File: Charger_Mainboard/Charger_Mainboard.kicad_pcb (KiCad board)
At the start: 2 copper layers, 100 x 100 mm, 57 parts, among them J1 Conn_01x02, J10 Conn_02x10_Odd_Even, J11 Conn_01x02_Pin, J12 Conn_01x02_Pin, J13 Conn_01x02_Pin, J14 Conn_01x02_Pin, J15 Conn_01x02_Pin, J16 Conn_01x02_Pin, J17 Conn_01x02_Pin, J18 Conn_01x04, J19 Conn_01x02_Pin, J2 Conn_01x02, J20 Conn_01x02_Pin, J21 Conn_01x04, J22 Conn_01x04, J23 Conn_01x02_Pin, J24 Conn_01x02_Pin, J3 Conn_01x02, J4 Conn_01x02, J5 Conn_01x02, J6 Conn_01x02, J7 Conn_01x02, J8 Conn_01x04, J9 Conn_01x02_Pin, U1 AP2204K-ADJ, U2 TLV2371DBV, U3 AP2204K-ADJ

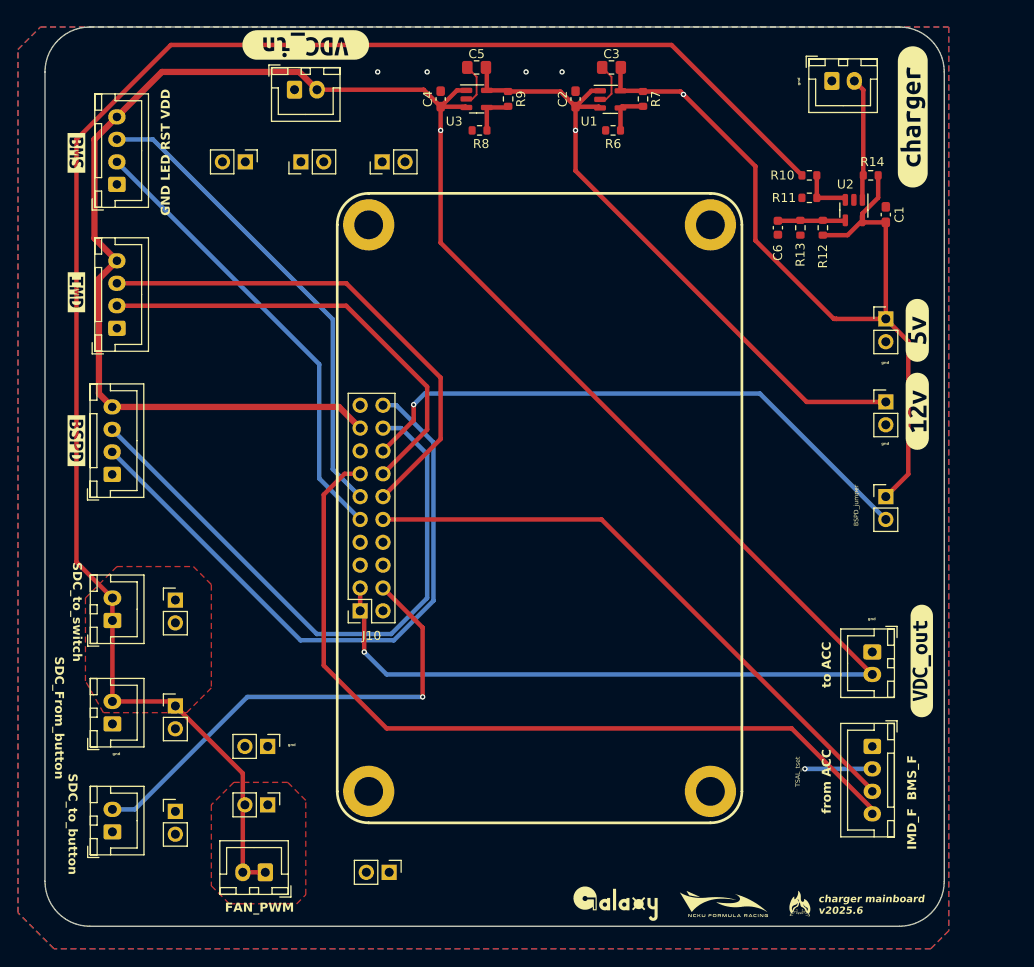
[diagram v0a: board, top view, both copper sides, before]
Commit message: Charger v2026.1
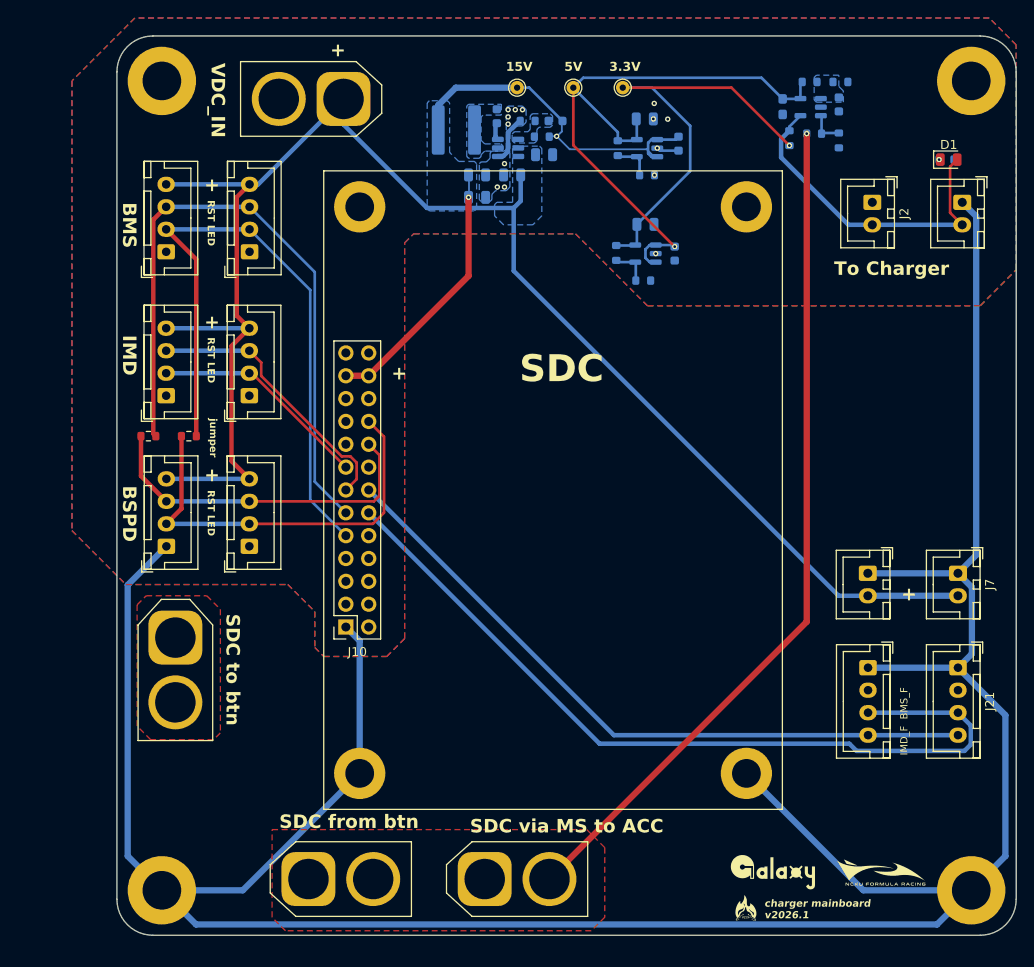
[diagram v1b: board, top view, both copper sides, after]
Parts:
- removed the H1 at (156.0, 65.0)
- removed the H2 at (118.0, 128.0)
- removed the H3 at (156.0, 128.0)
- removed the H4 at (118.0, 65.0)
- removed J11, J12, J13, J14, J15, J16, J17, J19, J20, J23, J24, J9: Conn_01x02_Pin, Connector_PinHeader_2.54mm:PinHeader_1x02_P2.54mm_Vertical
- removed the J18 at (90.0, 76.5)
- removed the J2 at (169.5, 49.0)
- removed the J21 at (174.0, 123.0)
- removed the J22 at (90.0, 60.5)
- removed J6: Conn_01x02, Connector_JST:JST_XH_B2B-XH-A_1x02_P2.50mm_Vertical
- removed the J7 at (174.0, 112.5)
- removed the J8 at (89.5, 92.8)
- removed kibuzzard-682D8AF9: G***, kibuzzard-682D8AF9
- removed kibuzzard-682D8B7A: G***, kibuzzard-682D8B7A
- removed kibuzzard-68452BF1: G***, kibuzzard-68452BF1
- removed kibuzzard-68452CD9: G***, kibuzzard-68452CD9
- removed kibuzzard-68452D38: G***, kibuzzard-68452D38
- removed kibuzzard-68452D90: G***, kibuzzard-68452D90
- removed kibuzzard-684531AC: G***, kibuzzard-684531AC
- removed kibuzzard-68453814: G***, kibuzzard-68453814
- added C10: 22u, Capacitor_SMD:C_0805_2012Metric, B.Cu at (130.1, 62.0)
- added C11: 1u, Capacitor_SMD:C_0603_1608Metric, B.Cu at (152.0, 68.2)
- added C12: 10u, Capacitor_SMD:C_0805_2012Metric, B.Cu at (148.8, 65.0)
- added C7: 100n, Capacitor_SMD:C_0603_1608Metric, B.Cu at (132.2, 52.9)
- added C8: 12p, Capacitor_SMD:C_0603_1608Metric, B.Cu at (138.8, 53.5)
- added C9: 22u, Capacitor_SMD:C_0805_2012Metric, B.Cu at (130.1, 59.5)
- added D1: LED_Small, LED_SMD:LED_0805_2012Metric, F.Cu at (182.5, 57.8)
- added H1: MountingHole_Pad, MountingHole:MountingHole_4.3mm_M4_ISO7380_Pad, F.Cu at (185.0, 49.0)
- added H1: MountingHole_Pad, MountingHole:MountingHole_3.2mm_M3_ISO7380_Pad, F.Cu at (160.0, 63.0)
- added H2: MountingHole_Pad, MountingHole:MountingHole_3.2mm_M3_ISO7380_Pad, F.Cu at (117.0, 126.0)
- added H2: MountingHole_Pad, MountingHole:MountingHole_4.3mm_M4_ISO7380_Pad, F.Cu at (185.0, 139.0)
- added H3: MountingHole_Pad, MountingHole:MountingHole_4.3mm_M4_ISO7380_Pad, F.Cu at (95.0, 49.0)
- added H3: MountingHole_Pad, MountingHole:MountingHole_3.2mm_M3_ISO7380_Pad, F.Cu at (160.0, 126.0)
- added H4: MountingHole_Pad, MountingHole:MountingHole_3.2mm_M3_ISO7380_Pad, F.Cu at (117.0, 63.0)
- added H4: MountingHole_Pad, MountingHole:MountingHole_4.3mm_M4_ISO7380_Pad, F.Cu at (95.0, 139.0)
- added J18: Conn_01x04, Connector_JST:JST_XH_B4B-XH-A_1x04_P2.50mm_Vertical, F.Cu at (104.7, 84.0)
- added J18: Conn_01x04, Connector_JST:JST_XH_B4B-XH-A_1x04_P2.50mm_Vertical, F.Cu at (95.5, 84.0)
- added J2: Conn_01x02, Connector_JST:JST_XH_B2B-XH-A_1x02_P2.50mm_Vertical, F.Cu at (174.0, 62.5)
- added J2: Conn_01x02, Connector_JST:JST_XH_B2B-XH-A_1x02_P2.50mm_Vertical, F.Cu at (184.0, 62.5)
- added J21: Conn_01x04, Connector_JST:JST_XH_B4B-XH-A_1x04_P2.50mm_Vertical, F.Cu at (183.5, 114.2)
- added J21: Conn_01x04, Connector_JST:JST_XH_B4B-XH-A_1x04_P2.50mm_Vertical, F.Cu at (173.5, 114.2)
- added J22: Conn_01x04, Connector_JST:JST_XH_B4B-XH-A_1x04_P2.50mm_Vertical, F.Cu at (104.8, 68.0)
- added J22: Conn_01x04, Connector_JST:JST_XH_B4B-XH-A_1x04_P2.50mm_Vertical, F.Cu at (95.5, 68.0)
- added J7: Conn_01x02, Connector_JST:JST_XH_B2B-XH-A_1x02_P2.50mm_Vertical, F.Cu at (183.5, 103.8)
- added J7: Conn_01x02, Connector_JST:JST_XH_B2B-XH-A_1x02_P2.50mm_Vertical, F.Cu at (173.5, 103.8)
- added J8: Conn_01x04, Connector_JST:JST_XH_B4B-XH-A_1x04_P2.50mm_Vertical, F.Cu at (95.5, 100.8)
- added J8: Conn_01x04, Connector_JST:JST_XH_B4B-XH-A_1x04_P2.50mm_Vertical, F.Cu at (104.7, 100.8)
- added L1: 15uH, Inductor_SMD:L_Coilcraft_XAL6060-XXX, B.Cu at (127.8, 54.5)
- added R1: 0, Resistor_SMD:R_0603_1608Metric, F.Cu at (93.5, 88.5)
- added R2: 0, Resistor_SMD:R_0603_1608Metric, F.Cu at (98.0, 88.5)
- added R3: 301k, Resistor_SMD:R_0603_1608Metric, B.Cu at (167.5, 54.9)
- added R4: 100k, Resistor_SMD:R_0603_1608Metric, B.Cu at (170.3, 55.6)
- added R5: 10k, Resistor_SMD:R_0603_1608Metric, B.Cu at (182.2, 57.8)
- added TP1: TestPoint, TestPoint:TestPoint_THTPad_D1.5mm_Drill0.7mm, F.Cu at (134.5, 49.8)
- added TP2: TestPoint, TestPoint:TestPoint_THTPad_D1.5mm_Drill0.7mm, F.Cu at (140.8, 49.8)
- added TP3: TestPoint, TestPoint:TestPoint_THTPad_D1.5mm_Drill0.7mm, F.Cu at (146.2, 49.8)
- added U4: AP2204K-ADJ, Package_TO_SOT_SMD:SOT-23-5, B.Cu at (148.8, 68.2)
- C1, C6, R12, R13, R14, R6, R7, U1: moved to B.Cu
- C2: footprint Capacitor_SMD:C_0603_1608Metric_Pad1.08x0.95mm_HandSolder -> Capacitor_SMD:C_0603_1608Metric; moved to B.Cu
- C3, C5: footprint Capacitor_SMD:C_0805_2012Metric_Pad1.18x1.45mm_HandSolder -> Capacitor_SMD:C_0805_2012Metric; moved to B.Cu
- C4: value 1u -> 10u; footprint Capacitor_SMD:C_0603_1608Metric_Pad1.08x0.95mm_HandSolder -> Capacitor_SMD:C_0805_2012Metric; moved to B.Cu
- J1, J3, J4, J5: footprint Connector_JST:JST_XH_B2B-XH-A_1x02_P2.50mm_Vertical -> Connector_AMASS:AMASS_XT60-M_1x02_P7.20mm_Vertical
- J10: value Conn_02x10_Odd_Even -> Conn_02x13_Odd_Even; footprint Connector_PinSocket_2.54mm:PinSocket_2x10_P2.54mm_Vertical -> Connector_PinSocket_2.54mm:PinSocket_2x13_P2.54mm_Vertical
- R10: value 100R -> 100k; moved to B.Cu
- R11: value 100k -> 165k; moved to B.Cu
- R8: value 100k -> 534k; moved to B.Cu
- R9: value 301k -> 30k1; moved to B.Cu
- U2: value TLV2371DBV -> AS331KTR-G1; moved to B.Cu
- U3: value AP2204K-ADJ -> AP63200WU; footprint Package_TO_SOT_SMD:SOT-23-5 -> Package_TO_SOT_SMD:TSOT-23-6; moved to B.Cu
- moved J5 50.4 mm to (130.9, 137.8), turned to 0 degrees
- moved J4 27.8 mm to (111.3, 137.8), turned to 0 degrees
- moved J3 22.7 mm to (96.5, 110.9), turned to -90 degrees
- moved R11 22.3 mm to (145.5, 68.1), turned to -90 degrees
- moved R10 21.9 mm to (148.5, 71.2), turned to 180 degrees
- moved G*** 17.8 mm to (175.0, 137.0)
- moved G*** 17.8 mm to (163.0, 137.0)
- moved R13 16.8 mm to (170.5, 49.1), turned to 0 degrees
- moved C1 16.6 mm to (164.0, 51.9), turned to -90 degrees
- moved R12 16.3 mm to (167.0, 49.1), turned to 0 degrees
- moved C6 15.3 mm to (170.3, 51.6)
- moved C4 13.1 mm to (137.5, 57.2), turned to 0 degrees
- moved C5 12.6 mm to (133.9, 59.5)
- moved C2 12.5 mm to (152.4, 56.0), turned to -90 degrees
- moved U2 12.4 mm to (167.1, 51.9), turned to 180 degrees
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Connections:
- C2 pad 1: +12V -> SDC_IN
- C4 pad 1: BSPD_IN -> VDC
- C5 pad 1: +12V -> VDC
- J1 pad 1: GND -> VDC
- J1 pad 2: BSPD_IN -> GND
- J10 pad 1: BSPD_IN -> GND
- J10 pad 10: BMS_FAULT -> SDC_OUT
- J10 pad 12: IMD_RST -> BMS_FAULT
- J10 pad 13: IMD_FAULT -> IMD_RST
- J10 pad 14: IMD_LED -> IMD_FAULT
- J10 pad 15: GND -> IMD_LED
- J10 pad 16: BSPD_FAULT -> unconnected-(J10-Pin_16-Pad16)
- J10 pad 17: BSPD_IN -> BSPD_FAULT
- J10 pad 2: GND -> unconnected-(J10-Pin_2-Pad2)
- J10 pad 3: BSPD_IN -> unconnected-(J10-Pin_3-Pad3)
- J10 pad 4: SDC_TO_SDBUTTON -> unconnected-(J10-Pin_4-Pad4)
- J10 pad 6: GND -> unconnected-(J10-Pin_6-Pad6)
- J10 pad 7: SW_Fault -> GND
- J3 pad 1: GND -> SDC_TO_SDBUTTON
- J4 pad 1: GND -> SDC_FROM_SDBUTTON
- J4 pad 2: FAN_PWM -> SDC_FROM_SDBUTTON
- J5 pad 1: FAN_PWM -> SDC_FROM_SDBUTTON
- J5 pad 2: FAN_PWM -> SDC_FROM_SDBUTTON
- R10 pad 1: FAN_PWM -> GND
- R10 pad 2: Net-(U2-+) -> Net-(U4-ADJ)
- R11 pad 1: Net-(U2-+) -> +3V3
- R11 pad 2: GND -> Net-(U4-ADJ)
- R14 pad 1: +5V -> +3V3
- R8 pad 1: GND -> SDC_IN
- R8 pad 2: Net-(U3-ADJ) -> Net-(U3-FB)
- R9 pad 1: +12V -> Net-(U3-FB)
- R9 pad 2: Net-(U3-ADJ) -> GND
- U1 pad 1: +12V -> SDC_IN
- U1 pad 3: +12V -> SDC_IN
- U2 pad 1: charger_analog -> Net-(U2--)
- U2 pad 4: Net-(U2--) -> charger_analog
- U3 pad 1: BSPD_IN -> Net-(U3-FB)
- U3 pad 2: GND -> VDC
- U3 pad 3: BSPD_IN -> VDC
- U3 pad 4: Net-(U3-ADJ) -> GND
- U3 pad 5: +12V -> Net-(U3-SW)
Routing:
- net GND: track 9.68 -> 320.3 mm, vias 4 -> 14
- net BSPD_IN: track 258.4 -> 0.00 mm, vias 2 -> 0
- net FAN_PWM: track 186.8 -> 0.00 mm
- net VDC: track 0.00 -> 178.7 mm
- net SDC_FROM_SDBUTTON: track 0.00 -> 94.7 mm, vias 0 -> 1
- net +12V: track 71.7 -> 0.00 mm, vias 1 -> 0
- net SDC_IN: track 0.00 -> 69.3 mm, vias 0 -> 2
- net BSPD_FAULT: track 65.4 -> 0.00 mm, vias 1 -> 0
- net SDC_TO_SDBUTTON: track 53.6 -> 0.00 mm, vias 1 -> 0
- net +3V3: track 0.00 -> 48.4 mm, vias 0 -> 1
- net BSPD_RST: track 68.2 -> 38.6 mm
- net BSPD_LED: track 71.8 -> 46.0 mm
- net IMD_LED: track 49.9 -> 24.3 mm
- net IMD_RST: track 56.2 -> 30.7 mm
- net BMS_FAULT: track 67.5 -> 92.3 mm
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- added copper zone on B.Cu, net Net-(U2--)
- added copper zone on B.Cu, net Net-(U3-FB)
- added copper zone on B.Cu, net Net-(U3-SW)
- added copper zone on F.Cu, net SDC_FROM_SDBUTTON
- added copper zone on B.Cu, net SDC_IN
- added copper zone on F.Cu, net SDC_TO_SDBUTTON
- added copper zone on B.Cu, net VDC
- removed copper zone on F.Cu, net FAN_PWM
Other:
- outline, holes or cut-outs redrawn
- board text added: "+"
- board text added: "15V"
- board text added: "3.3V"
- board text added: "5V"
- board text added: "BMS"
- board text added: "BSPD"
- board text added: "IMD"
- board text added: "LED"
- board text added: "RST"
- board text added: "SDC"
- board text added: "SDC from btn"
- board text added: "SDC to btn"
- board text added: "SDC via MS to ACC"
- board text added: "To Charger"
- board text added: "VDC_IN"
- board text added: "charger mainboard v2026.1"
- board text added: "jumper"
- board text removed: "BSPD_jumper"
- board text removed: "FAN_PWM"
- board text removed: "GND LED RST VDD"
- board text removed: "SDC_From_button"
- board text removed: "SDC_to_button"
- board text removed: "SDC_to_switch"
- board text removed: "TSAL_tset"
- board text removed: "charger mainboard v2025.6"
- board text removed: "from ACC"
- board text removed: "gnd"
- board text removed: "to ACC"
